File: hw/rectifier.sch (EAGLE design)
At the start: 78 parts

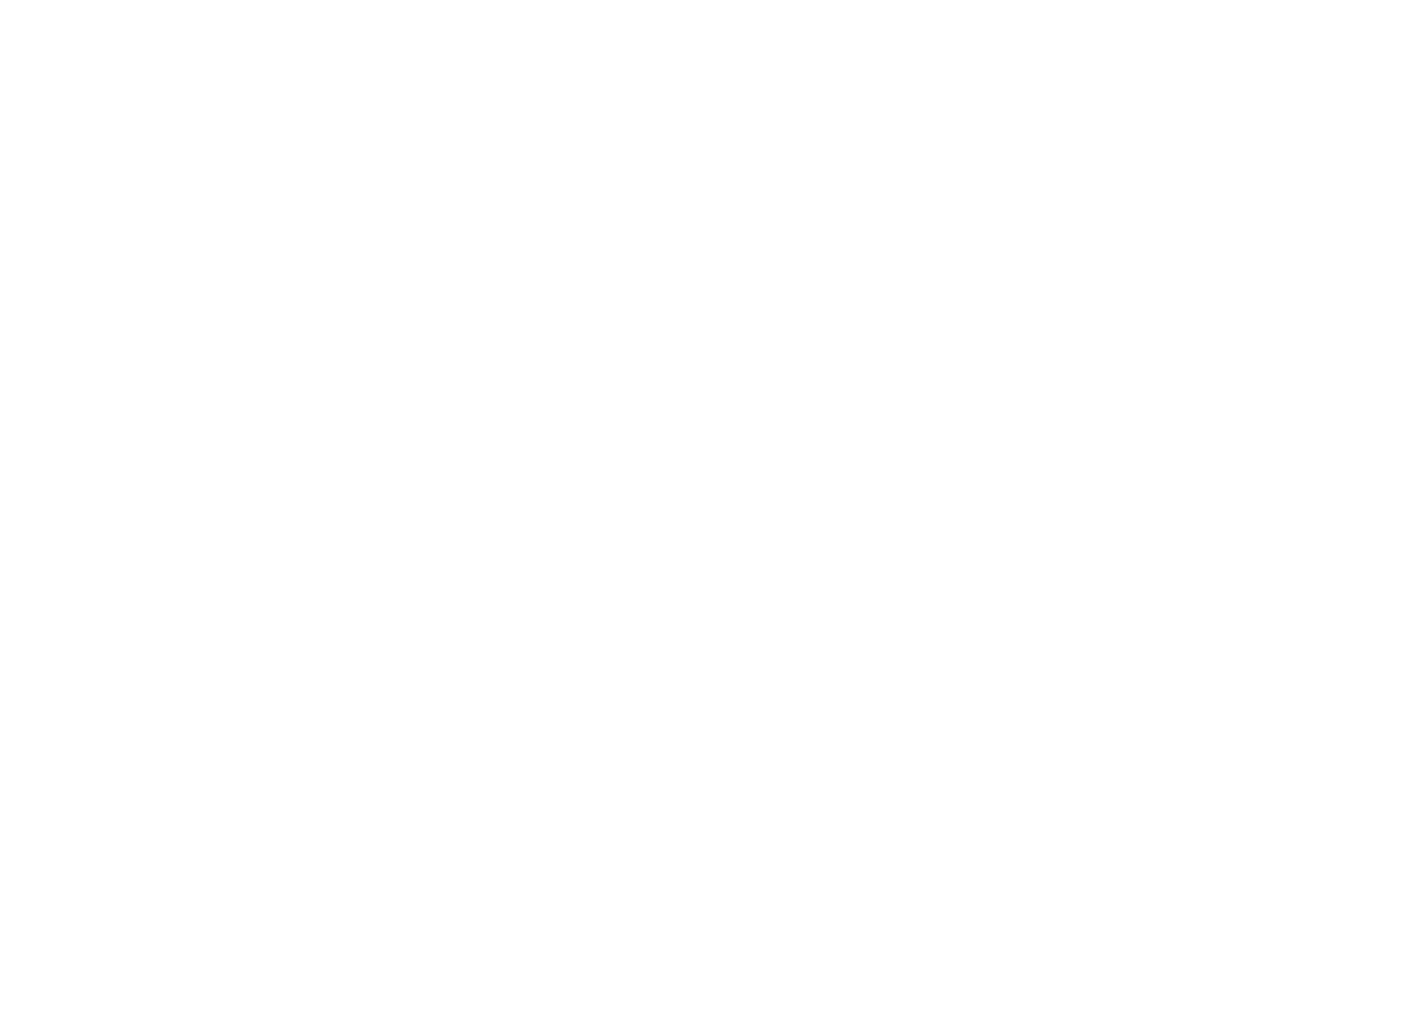
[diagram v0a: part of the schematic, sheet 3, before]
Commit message: Add loop section: wip
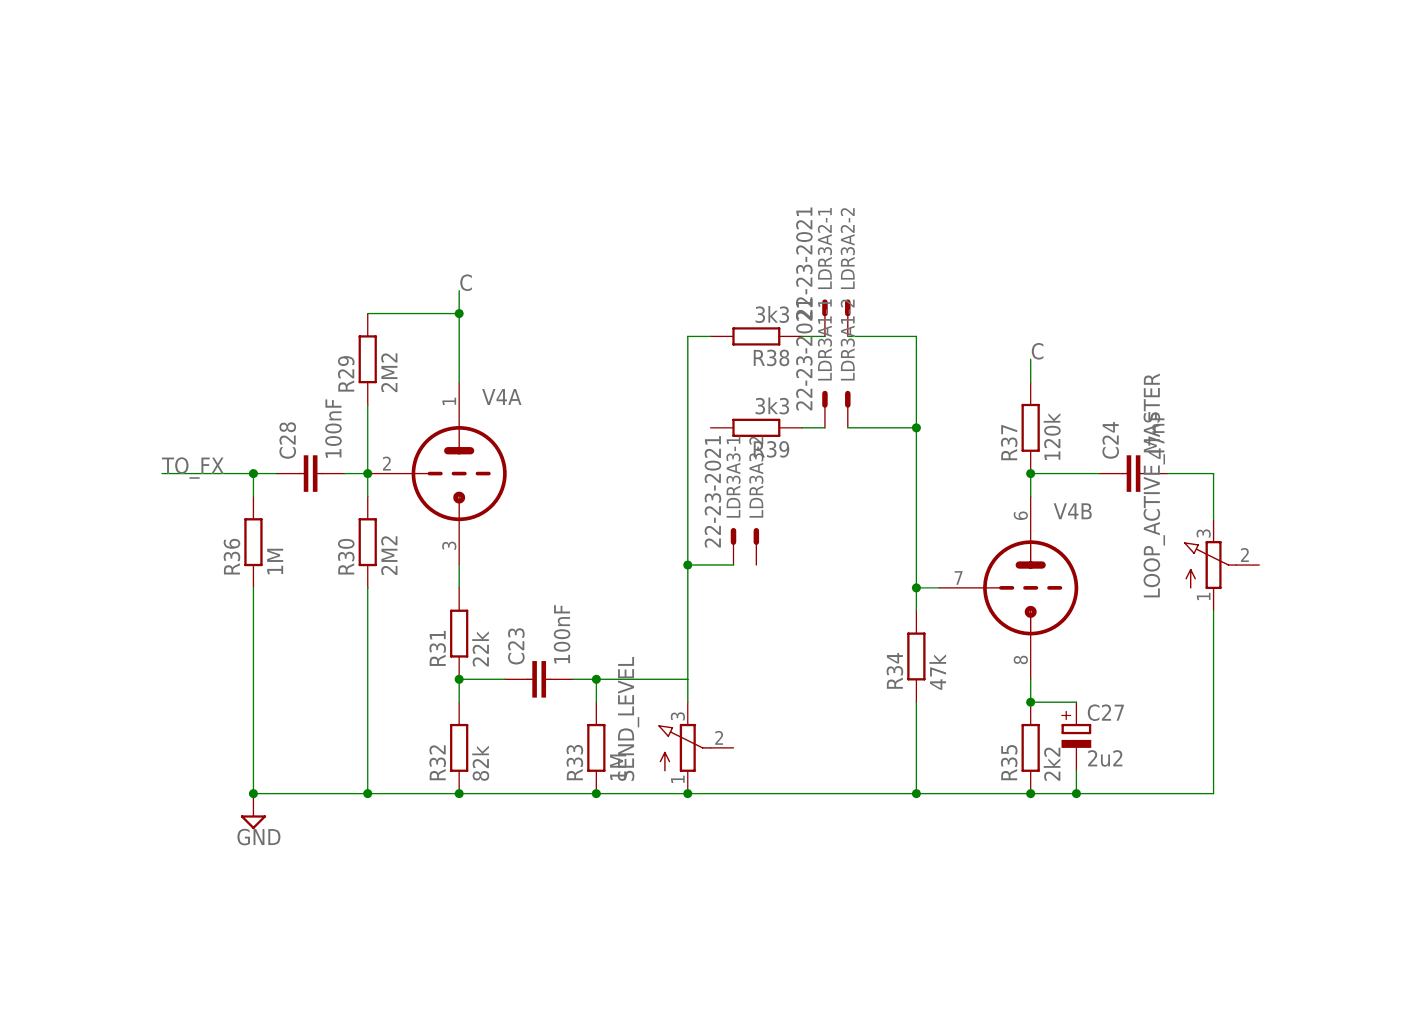
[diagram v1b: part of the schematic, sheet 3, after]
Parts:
- added C23, C28: 100nF, capacitor-wima:C7.5/5
- added C24: 47nF, capacitor-wima:C7.5/5
- added C27: 2u2, rcl:CPOL-EUE3.5-8
- added LDR3A1, LDR3A2, LDR3A3: 22-23-2021, con-molex:22-23-2021
- added LOOP_ACTIVE_MASTER, SEND_LEVEL: (no value), pot:3RP/1610N
- added R29, R30: 2M2, rcl:R-EU_0207/10
- added R31: 22k, rcl:R-EU_0207/10
- added R32: 82k, rcl:R-EU_0207/10
- added R33, R36: 1M, rcl:R-EU_0207/10
- added R34: 47k, rcl:R-EU_0207/10
- added R35: 2k2, rcl:R-EU_0207/10
- added R37: 120k, rcl:R-EU_0207/10
- added R38, R39: 3k3, rcl:R-EU_0207/10
- added V4: (no value), tubes:12AX7-P
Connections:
- new net N$43: C28.2, R29.1, R30.2, V4A.TG
- new net N$44: LDR3A1-2.S, LDR3A2-2.S, R34.2, V4B.TG
- new net N$45: R31.2, V4A.TK
- new net N$46: C23.1, R31.1, R32.2
- new net N$47: C23.2, LDR3A3-1.S, R33.2, R38.2, SEND_LEVEL.E
- new net N$48: C27.+, R35.2, V4B.TK
- new net N$49: C24.1, R37.1, V4B.TA
- new net N$50: LDR3A2-1.S, R38.1
- new net N$51: C24.2, LOOP_ACTIVE_MASTER.E
- new net N$52: LDR3A1-1.S, R39.1
- net C: now also R29.2, R37.2, V4A.TA
- net GND: now also C27.-, LOOP_ACTIVE_MASTER.A, R30.1, R32.1, R33.1, R34.1, R35.1, R36.1, SEND_LEVEL.A
- net TO_FX: now also C28.1, R36.2

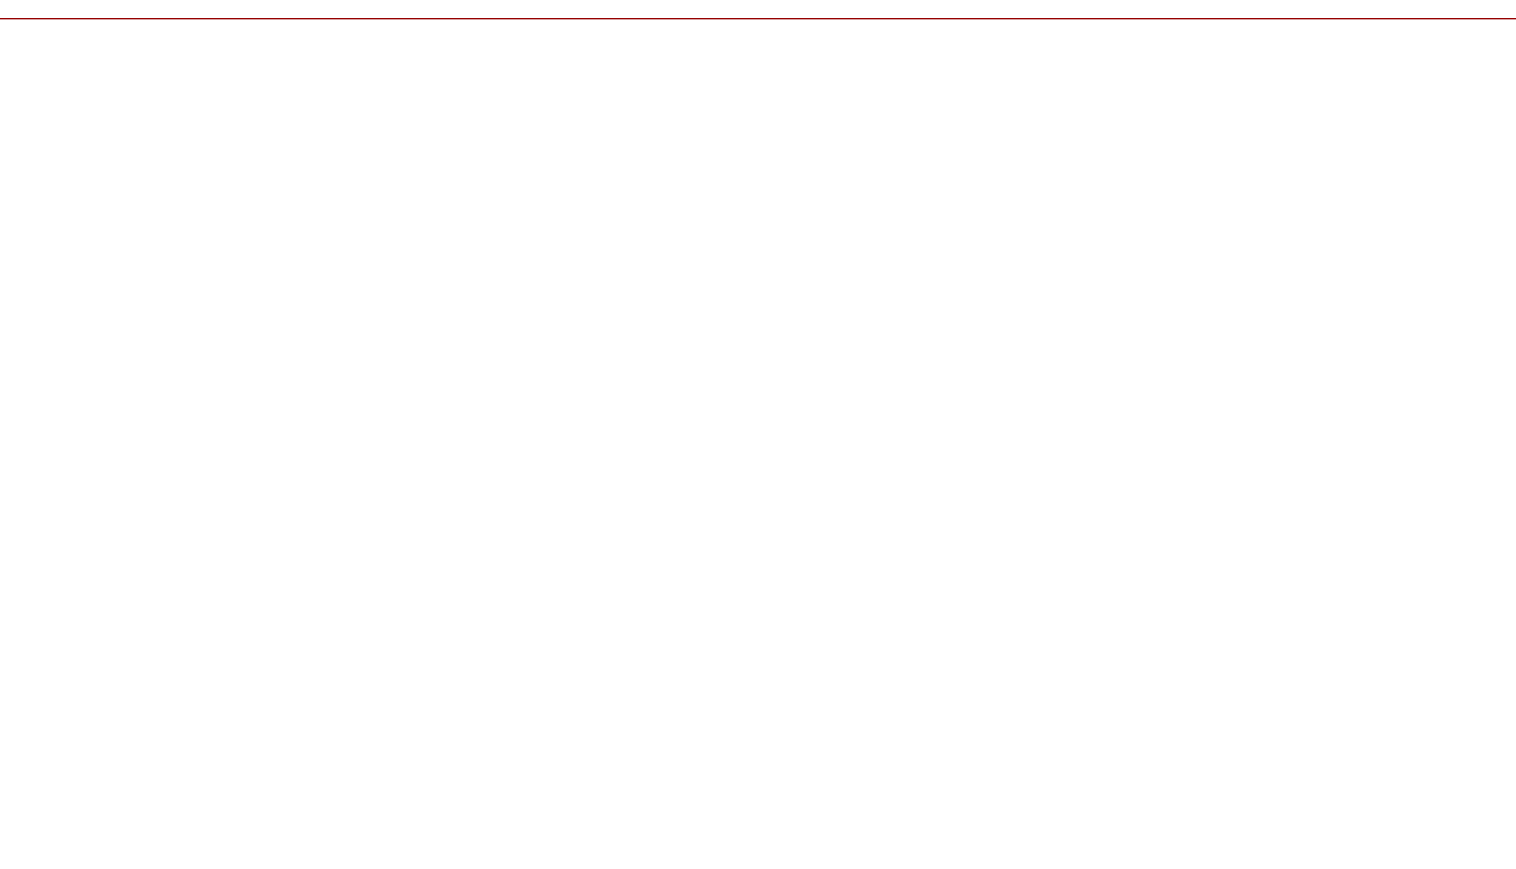
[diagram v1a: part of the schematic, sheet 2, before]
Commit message: Start power section
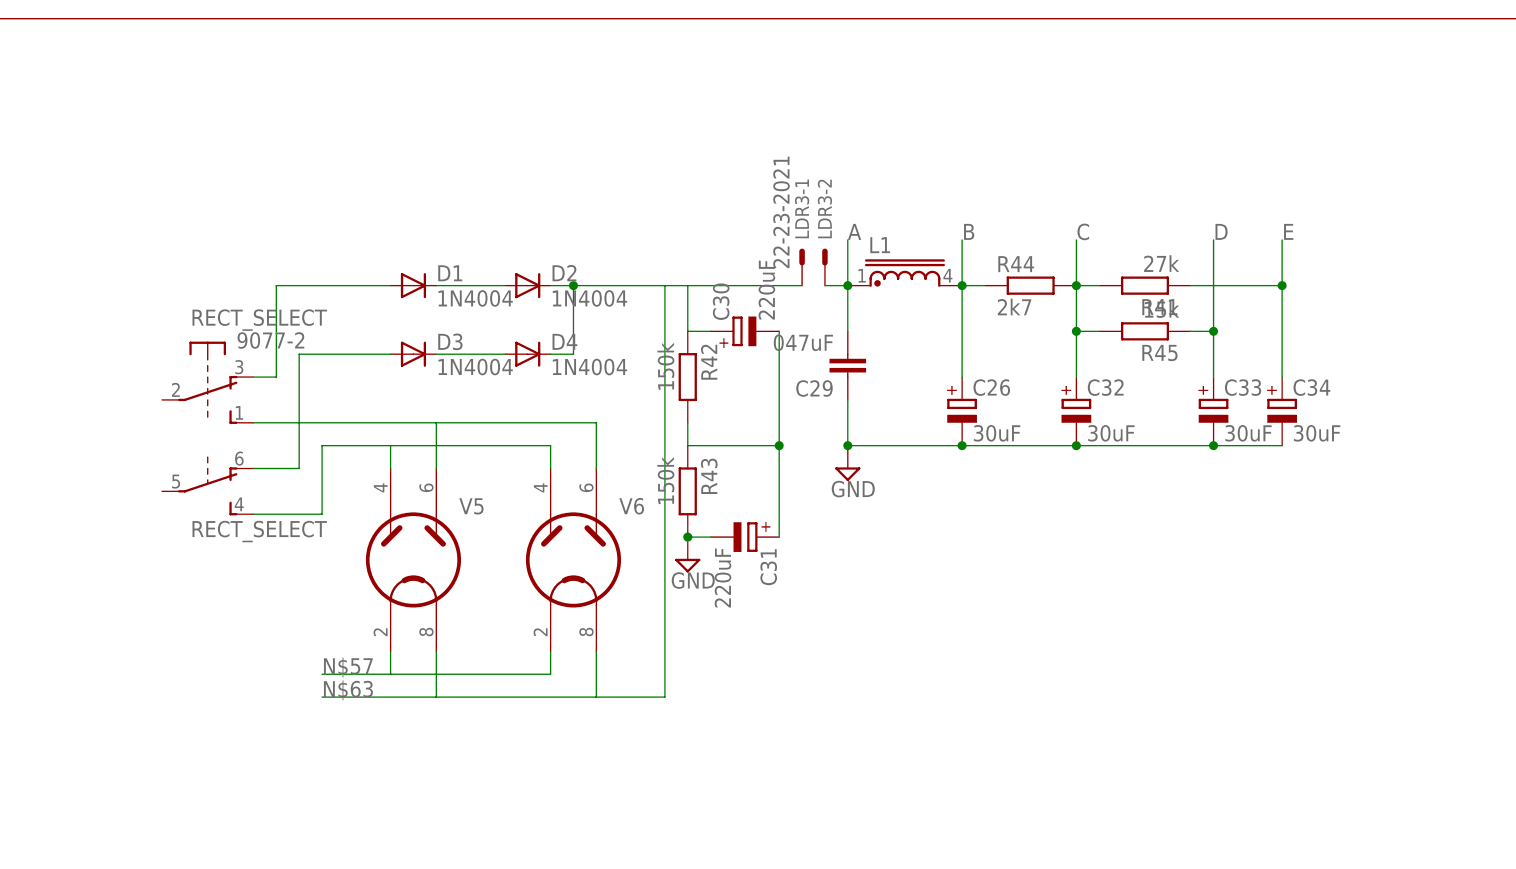
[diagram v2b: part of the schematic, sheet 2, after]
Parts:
- added C26, C32, C33, C34: 30uF, rcl:CPOL-EUE3.5-8
- added C29: 047uF, capacitor-wima:C7.5/5
- added C30, C31: 220uF, rcl:CPOL-EUE3.5-8
- added D1, D2, D3, D4: 1N4004, diode:1N4004
- added L1: (no value), inductor-neosid:U15-CHOKE
- added LDR3: 22-23-2021, con-molex:22-23-2021
- added R41: 27k, rcl:R-EU_0207/10
- added R42, R43: 150k, rcl:R-EU_0207/10
- added R44: 2k7, rcl:R-EU_0207/10
- added R45: 15k, rcl:R-EU_0207/10
- added RECT_SELECT: 9077-2, switch-misc:9077-2
- added V5, V6: (no value), tubes:5U4GB
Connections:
- new net A: C29.2, L1.1, LDR3-2.S
- new net B: C26.+, L1.4, R44.1
- new net N$53: D1.C, D2.A
- new net N$54: D3.C, D4.A
- new net N$56: C30.-, C31.+, R42.2, R43.1
- new net N$57: V5.H1, V6.H1
- new net N$58: RECT_SELECT2.S, V5.A1, V6.A1
- new net N$59: RECT_SELECT1.S, V5.A2, V6.A2
- new net N$60: D3.A, RECT_SELECT2.O
- new net N$61: D1.A, RECT_SELECT1.O
- new net N$63: C30.+, D2.C, D4.C, LDR3-1.S, R42.1, V5.H2, V6.H2
- net C: now also C32.+, R41.2, R44.2, R45.2
- net D: now also C33.+, R45.1
- net E: now also C34.+, R41.1
- net GND: now also C26.-, C29.1, C31.-, C32.-, C33.-, C34.-, R43.2
